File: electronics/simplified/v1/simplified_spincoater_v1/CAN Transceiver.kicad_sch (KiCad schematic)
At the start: 2 parts, among them U18 TJA1051TK/3

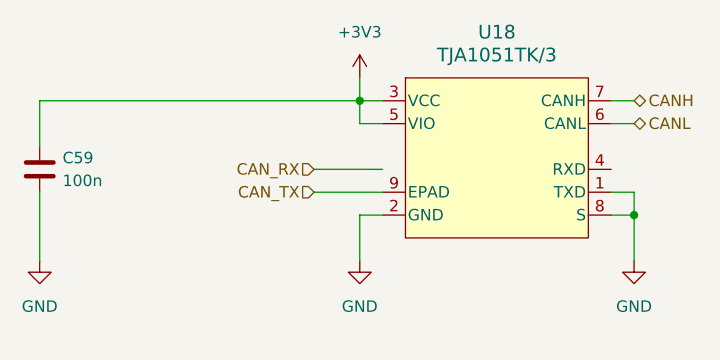
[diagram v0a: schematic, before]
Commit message: fix
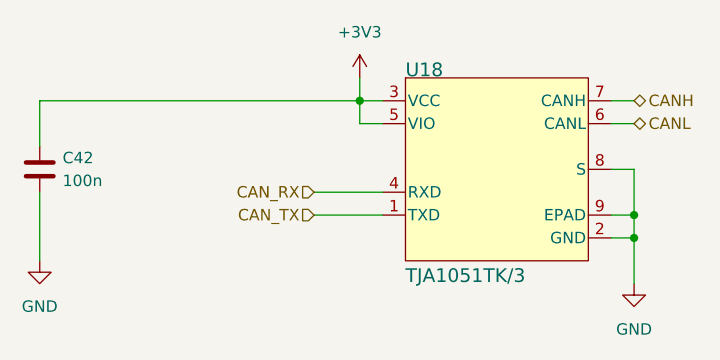
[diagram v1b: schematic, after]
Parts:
- removed C59: 100n, Capacitor_SMD:C_0402_1005Metric, symbol Device:C
- added C42: 100n, Capacitor_SMD:C_0402_1005Metric, symbol Device:C
- U18: Manufacturer (none) -> NXP Semicon; Manufacturer Part Number (none) -> TJA1051TK/3
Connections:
- net +3V3: now also C42.1
- net CAN_RX: now also U18.4 (RXD)
- net CAN_TX: now also U18.1 (TXD); no longer U18.9 (EPAD)
- net GND: now also U18.9 (EPAD), C42.2; no longer U18.1 (TXD)
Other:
- moved on the sheet: U18
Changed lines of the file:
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@@
 	(paper "A4")
+	(junction
+		(at 167.64 99.06)
+		(diameter 0)
+		(color 0 0 0 0)
+	)
 	(junction
 		(at 137.16 83.82)
@@
 	(wire
 		(pts
-			(xy 167.64 93.98) (xy 167.64 96.52)
+			(xy 167.64 96.52) (xy 167.64 99.06)
 		)
 		(stroke
@@
 	(wire
 		(pts
+			(xy 132.08 96.52) (xy 139.7 96.52)
+		)
+		(stroke
+			(width 0)
+			(type default)
+		)
+	)
+	(wire
+		(pts
+			(xy 101.6 93.98) (xy 101.6 101.6)
+		)
+		(stroke
+			(width 0)
+			(type default)
+		)
+	)
+	(wire
+		(pts
+			(xy 137.16 83.82) (xy 137.16 86.36)
+		)
+		(stroke
+			(width 0)
+			(type default)
+		)
+	)
+	(wire
+		(pts
+			(xy 165.1 99.06) (xy 167.64 99.06)
+		)
+		(stroke
+			(width 0)
+			(type default)
+		)
+	)
+	(wire
+		(pts
+			(xy 101.6 83.82) (xy 137.16 83.82)
+		)
+		(stroke
+			(width 0)
+			(type default)
+		)
+	)
+	(wire
+		(pts
+			(xy 101.6 83.82) (xy 101.6 88.9)
+		)
+		(stroke
+			(width 0)
+			(type default)
+		)
+	)
+	(wire
+		(pts
+			(xy 165.1 91.44) (xy 167.64 91.44)
+		)
+		(stroke
+			(width 0)
+			(type default)
+		)
+	)
+	(wire
+		(pts
 			(xy 132.08 93.98) (xy 139.7 93.98)
 		)
@@
 	(wire
 		(pts
-			(xy 137.16 96.52) (xy 139.7 96.52)
-		)
-		(stroke
-			(width 0)
-			(type default)
-		)
-	)
-	(wire
-		(pts
-			(xy 101.6 93.98) (xy 101.6 101.6)
-		)
-		(stroke
-			(width 0)
-			(type default)
-		)
-	)
-	(wire
-		(pts
-			(xy 137.16 83.82) (xy 137.16 86.36)
-		)
-		(stroke
-			(width 0)
-			(type default)
-		)
-	)
-	(wire
-		(pts
-			(xy 165.1 93.98) (xy 167.64 93.98)
-		)
-		(stroke
-			(width 0)
-			(type default)
-		)
-	)
-	(wire
-		(pts
-			(xy 101.6 83.82) (xy 137.16 83.82)
-		)
-		(stroke
-			(width 0)
-			(type default)
-		)
-	)
-	(wire
-		(pts
-			(xy 101.6 83.82) (xy 101.6 88.9)
-		)
-		(stroke
-			(width 0)
-			(type default)
-		)
-	)
-	(wire
-		(pts
-			(xy 132.08 91.44) (xy 139.7 91.44)
-		)
-		(stroke
-			(width 0)
-			(type default)
-		)
-	)
-	(wire
-		(pts
 			(xy 137.16 83.82) (xy 137.16 81.28)
 		)
@@
 	(wire
 		(pts
+			(xy 165.1 86.36) (xy 167.64 86.36)
+		)
+		(stroke
+			(width 0)
+			(type default)
+		)
+	)
+	(wire
+		(pts
 			(xy 165.1 96.52) (xy 167.64 96.52)
 		)
@@
 	(wire
 		(pts
-			(xy 165.1 86.36) (xy 167.64 86.36)
-		)
-		(stroke
-			(width 0)
-			(type default)
-		)
-	)
-	(wire
-		(pts
-			(xy 167.64 96.52) (xy 167.64 101.6)
-		)
-		(stroke
-			(width 0)
-			(type default)
-		)
-	)
-	(wire
-		(pts
 			(xy 165.1 83.82) (xy 167.64 83.82)
 		)
@@
 	(wire
 		(pts
-			(xy 137.16 101.6) (xy 137.16 96.52)
+			(xy 167.64 96.52) (xy 167.64 91.44)
+		)
+		(stroke
+			(width 0)
+			(type default)
+		)
+	)
+	(wire
+		(pts
+			(xy 167.64 99.06) (xy 167.64 104.14)
 		)
 		(stroke
@@
 	(hierarchical_label "CAN_RX"
 		(shape input)
-		(at 132.08 91.44 180)
+		(at 132.08 93.98 180)
 		(effects
 			(font
@@
 	(hierarchical_label "CAN_TX"
 		(shape input)
-		(at 132.08 93.98 180)
+		(at 132.08 96.52 180)
 		(effects
 			(font
@@
 	(symbol
 		(lib_id "power:GND")
-		(at 167.64 101.6 0)
+		(at 167.64 104.14 0)
 		(unit 1)
 		(exclude_from_sim no)
@@
 		(fields_autoplaced yes)
 		(property "Reference" "#PWR0119"
-			(at 167.64 107.95 0)
+			(at 167.64 110.49 0)
 			(effects
 				(font
@@
 		)
 		(property "Value" "GND"
-			(at 167.64 106.68 0)
+			(at 167.64 109.22 0)
 			(effects
 				(font
@@
 		)
 		(property "Footprint" ""
-			(at 167.64 101.6 0)
+			(at 167.64 104.14 0)
 			(effects
 				(font
@@
 		)
 		(property "Datasheet" ""
-			(at 167.64 101.6 0)
+			(at 167.64 104.14 0)
 			(effects
 				(font
@@
 		)
 		(property "Description" "Power symbol creates a global label with name \"GND\" , ground"
-			(at 167.64 101.6 0)
+			(at 167.64 104.14 0)
 			(effects
 				(font
@@
 				(path "/82f7d8d0-a6dd-48aa-80fa-49fc2cccb16f/51a0530e-a541-446c-8cbb-8049bd9a895b"
 					(reference "#PWR0120")
-					(unit 1)
-				)
-			)
-		)
-	)
-	(symbol
-		(lib_id "power:GND")
-		(at 137.16 101.6 0)
-		(unit 1)
-		(exclude_from_sim no)
-		(in_bom yes)
-		(on_board yes)
-		(dnp no)
-		(fields_autoplaced yes)
-		(property "Reference" "#PWR0118"
-			(at 137.16 107.95 0)
-			(effects
-				(font
-					(size 1.27 1.27)
-				)
-				(hide yes)
-			)
-		)
-		(property "Value" "GND"
-			(at 137.16 106.68 0)
-			(effects
-				(font
-					(size 1.27 1.27)
-				)
-			)
-		)
-		(property "Footprint" ""
-			(at 137.16 101.6 0)
-			(effects
-				(font
-					(size 1.27 1.27)
-				)
-				(hide yes)
-			)
-		)
-		(property "Datasheet" ""
-			(at 137.16 101.6 0)
-			(effects
-				(font
-					(size 1.27 1.27)
-				)
-				(hide yes)
-			)
-		)
-		(property "Description" "Power symbol creates a global label with name \"GND\" , ground"
-			(at 137.16 101.6 0)
-			(effects
-				(font
-					(size 1.27 1.27)
-				)
-				(hide yes)
-			)
-		)
-		(pin "1"
-		)
-		(instances
-			(project "simplified_spincoater_v1"
-				(path "/82f7d8d0-a6dd-48aa-80fa-49fc2cccb16f/1b9d8d50-bf31-43c5-a329-47671a272977"
-					(reference "#PWR0118")
-					(unit 1)
-				)
-				(path "/82f7d8d0-a6dd-48aa-80fa-49fc2cccb16f/51a0530e-a541-446c-8cbb-8049bd9a895b"
-					(reference "#PWR019")
 					(unit 1)
 				)
@@
 		(on_board yes)
 		(dnp no)
-		(fields_autoplaced yes)
 		(property "Reference" "U18"
-			(at 152.4 76.2 0)
+			(at 142.24 81.28 0)
 			(effects
 				(font
 					(size 1.524 1.524)
 				)
+				(justify left bottom)
 			)
 		)
 		(property "Value" "TJA1051TK/3"
-			(at 152.4 78.74 0)
+			(at 142.24 104.14 0)
 			(effects
 				(font
 					(size 1.524 1.524)
 				)
+				(justify left bottom)
 			)
 		)
@@
 		)
 		(property "Description" ""
+			(at 142.24 81.28 0)
+			(effects
+				(font
+					(size 1.27 1.27)
+				)
+				(hide yes)
+			)
+		)
+		(property "Manufacturer" "NXP Semicon"
+			(at 142.24 81.28 0)
+			(effects
+				(font
+					(size 1.27 1.27)
+				)
+				(hide yes)
+			)
+		)
+		(property "Manufacturer Part Number" "TJA1051TK/3"
 			(at 142.24 81.28 0)
 			(effects
@@
 		(dnp no)
 		(fields_autoplaced yes)
-		(property "Reference" "C59"
+		(property "Reference" "C42"
 			(at 104.14 90.1699 0)
 			(effects
@@
 			)
 		)
-		(property "Description" "Unpolarized capacitor"
+		(property "Description" "MLCC"
+			(at 101.6 91.44 0)
+			(effects
+				(font
+					(size 1.27 1.27)
+				)
+				(hide yes)
+			)
+		)
+		(property "Manufacturer" "Murata Electronics"
+			(at 101.6 91.44 0)
+			(effects
+				(font
+					(size 1.27 1.27)
+				)
+				(hide yes)
+			)
+		)
+		(property "Manufacturer Part Number" "GRM155R62A104ME14D"
 			(at 101.6 91.44 0)
 			(effects
@@
 			(project "simplified_spincoater_v1"
 				(path "/82f7d8d0-a6dd-48aa-80fa-49fc2cccb16f/1b9d8d50-bf31-43c5-a329-47671a272977"
-					(reference "C59")
+					(reference "C42")
 					(unit 1)
 				)
 				(path "/82f7d8d0-a6dd-48aa-80fa-49fc2cccb16f/51a0530e-a541-446c-8cbb-8049bd9a895b"
-					(reference "C32")
-					(unit 1)
-				)
+					(reference "C43")
+					(unit 1)
+				)
